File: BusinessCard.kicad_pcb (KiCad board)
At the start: 2 copper layers, 88.9 x 50.8 mm, 7 parts, among them Q1 Q_NMOS_DGS

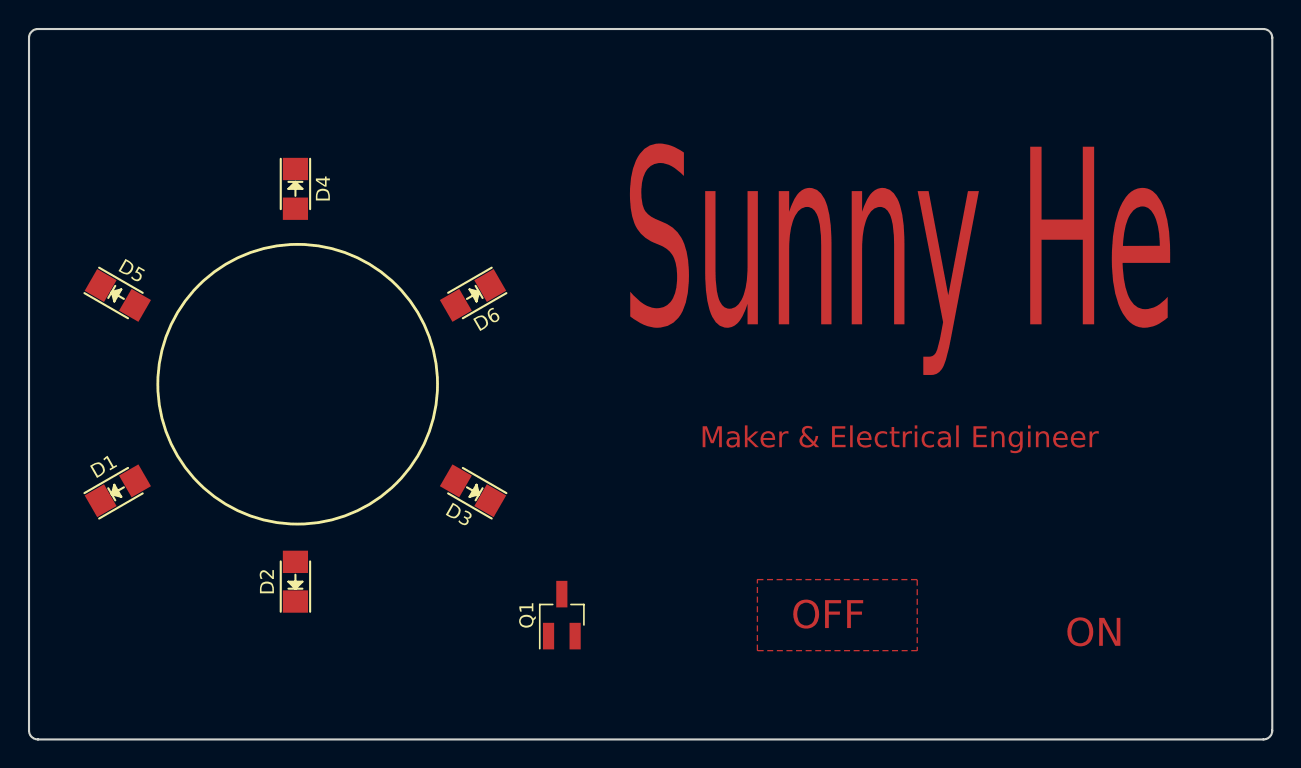
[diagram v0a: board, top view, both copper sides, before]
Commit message: First draft of front
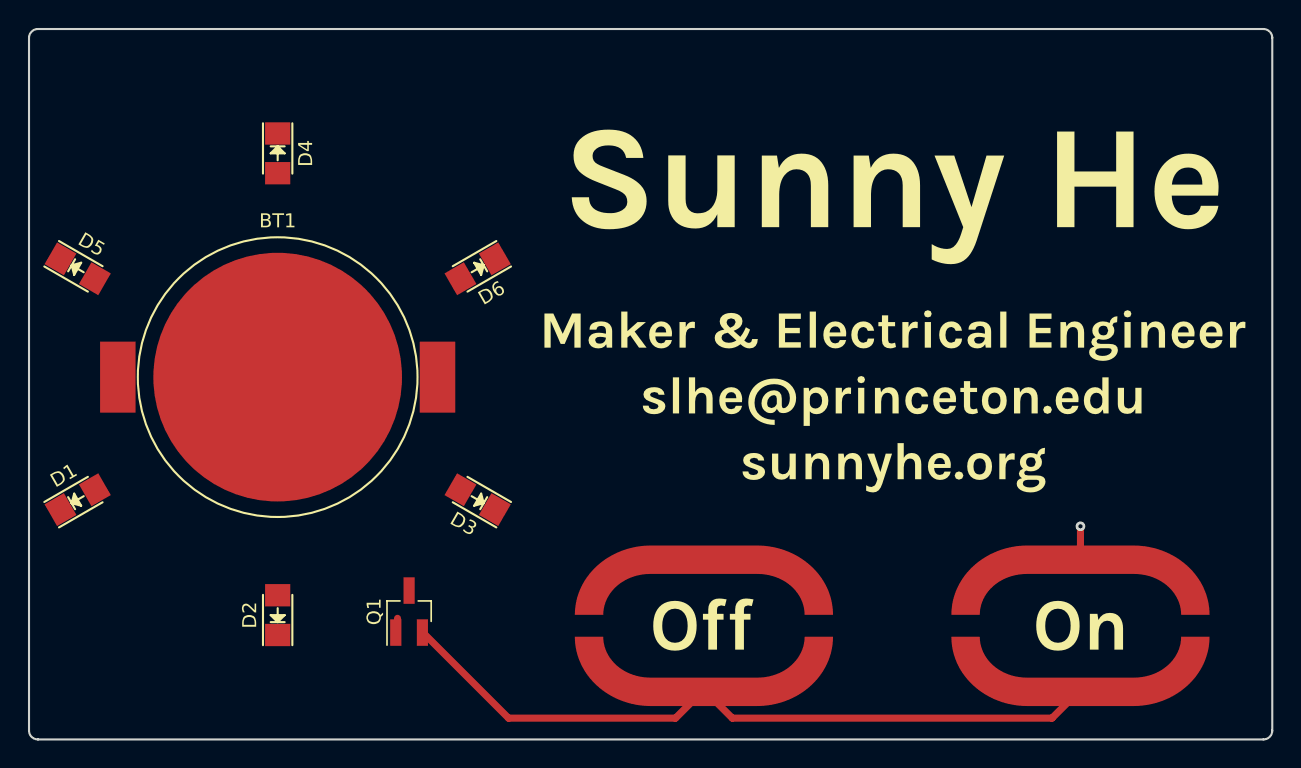
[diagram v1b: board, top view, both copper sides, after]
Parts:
- added BT1: Battery_Cell, CardElements:Linx_CR2032_Holder, F.Cu at (68.6, 75.7)
- added P1: ButtonPad, CardElements:ButtonPad, F.Cu at (99.1, 96.8)
- added P2: ButtonPad, CardElements:ButtonPad, F.Cu at (99.1, 90.2)
- added P3: ButtonPad, CardElements:ButtonPad, F.Cu at (126.0, 96.8)
- added P4: ButtonPad, CardElements:ButtonPad, F.Cu at (126.0, 90.2)
- added svg2mod: G***, CardElements:front, F.Cu at (92.7, 72.4)
- moved Q1 10.9 mm to (78.0, 92.5)
- moved D5 3.44 mm to (54.3, 67.9)
- moved D1 2.94 mm to (54.3, 84.5)
- moved D4 2.84 mm to (68.6, 59.7)
- moved D2 2.71 mm to (68.6, 92.7)
- moved D6 1.93 mm to (82.9, 67.9)
- moved D3 0.72 mm to (82.9, 84.5)
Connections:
- net Net-(BT1-Pad1) renamed +3V3
- net Net-(D1-Pad1) renamed Cathode
- Q1 pad 2: Net-(Q1-Pad2) -> Sense
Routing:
- net Sense: track 0.00 -> 52.6 mm
- net +3V3: track 0.00 -> 2.54 mm, vias 0 -> 1
- removed copper zone on F.Cu, net GND
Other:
- net class Default: clearance 0.2 -> 0.254; trace_width 0.25 -> 0.508; via_dia 0.6 -> 0.6858; via_drill 0.4 -> 0.3048
- rule trace_clearance: 0.2 -> 0.254
- board text removed: "Maker & Electrical Engineer"
- board text removed: "OFF"
- board text removed: "ON"
- board text removed: "Sunny He"
